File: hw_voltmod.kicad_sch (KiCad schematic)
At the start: 10 parts, among them J101 Conn_01x09_Pin, U104 L78L33_SO8

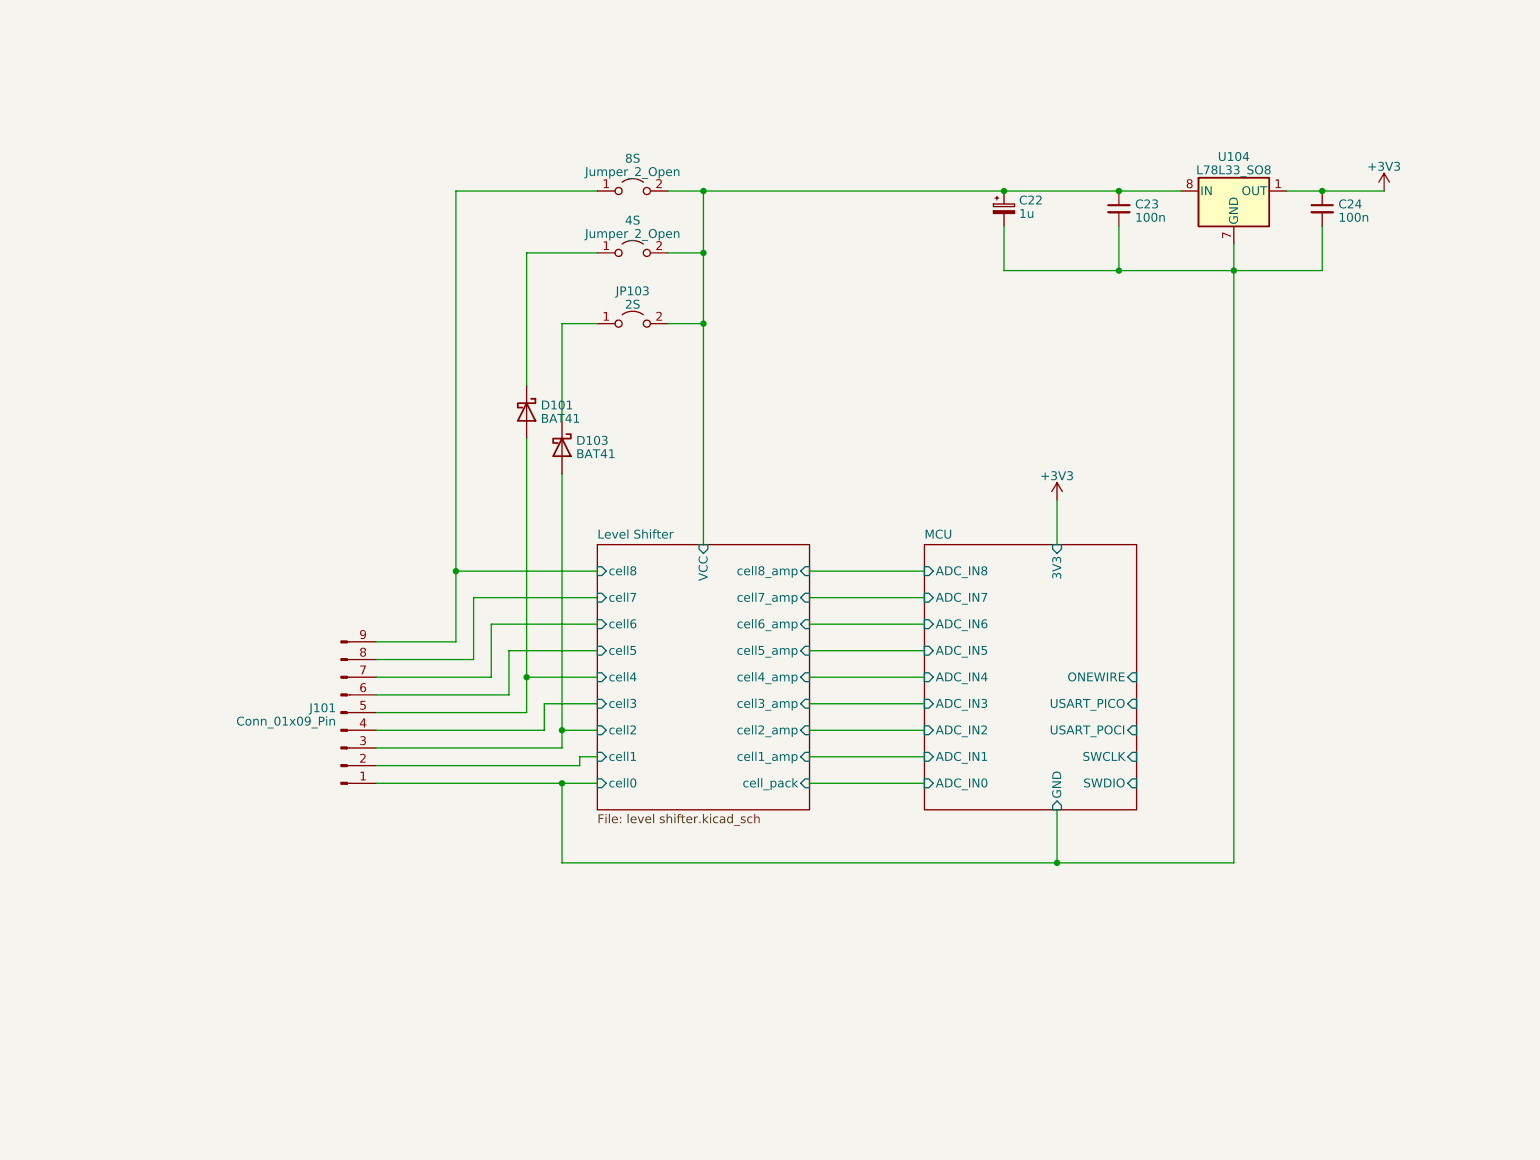
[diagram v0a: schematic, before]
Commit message: asdf
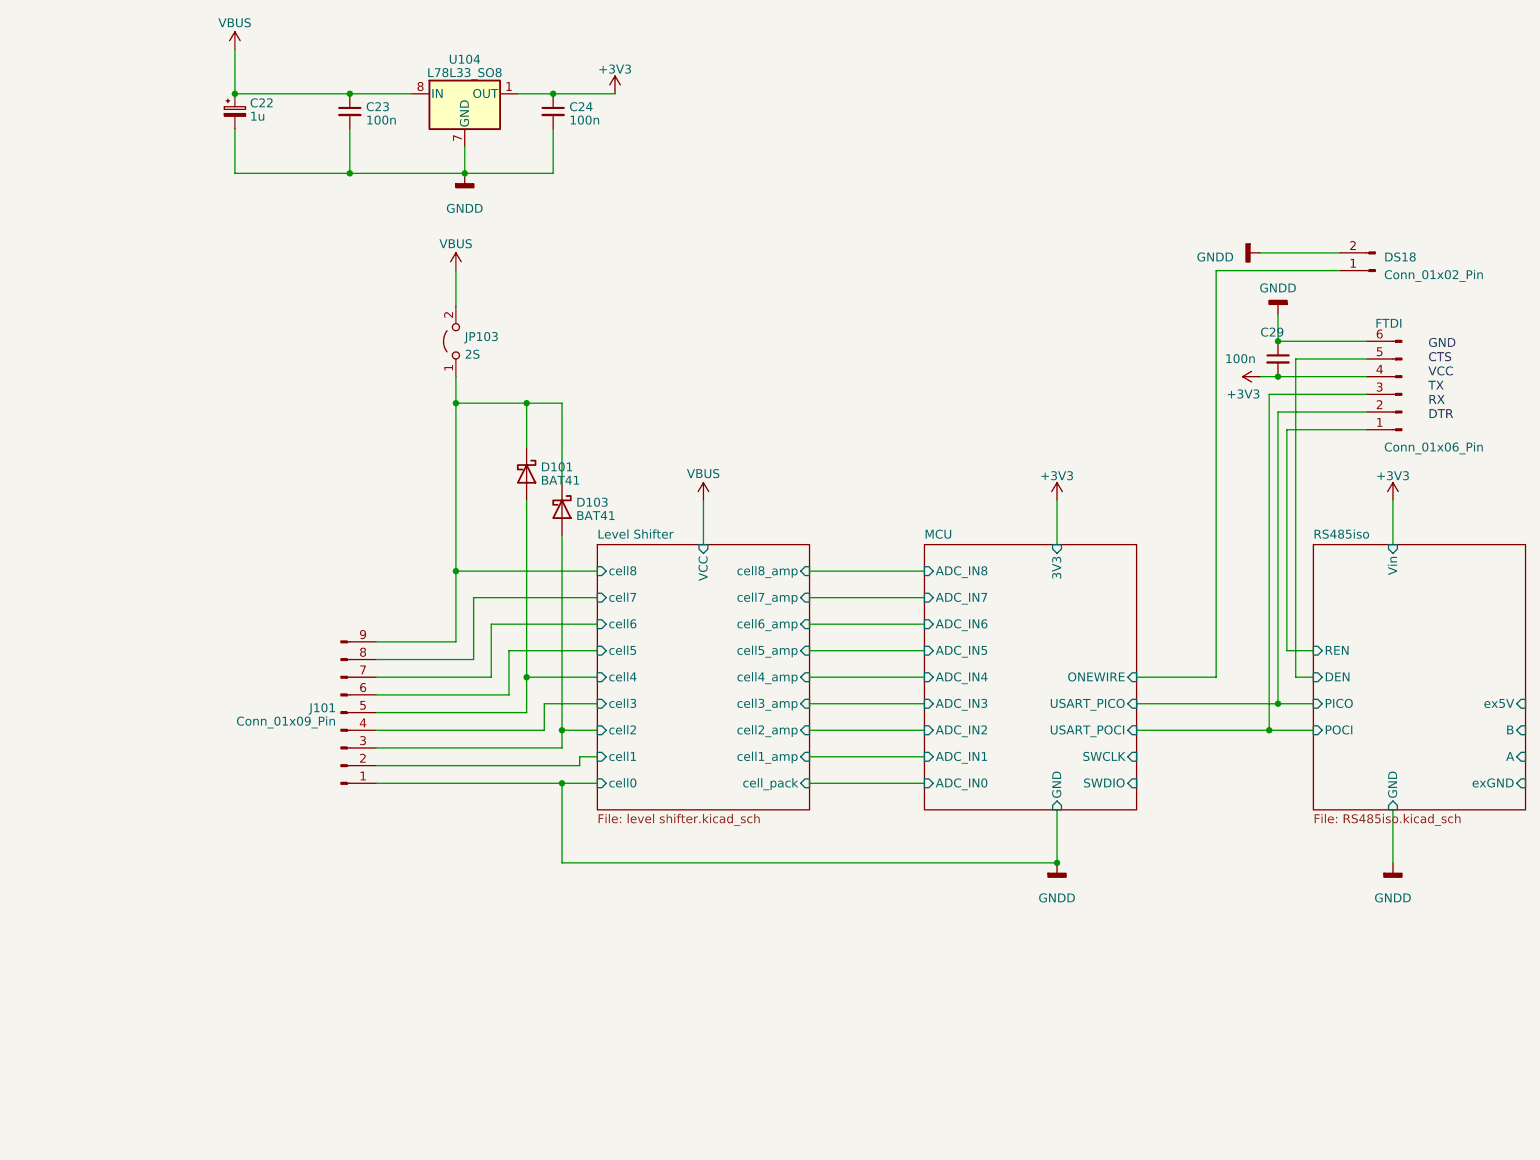
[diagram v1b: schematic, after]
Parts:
- removed 4S, 8S: Jumper_2_Open, symbol Jumper:Jumper_2_Open
- added C29: 100n, Capacitor_SMD:C_0603_1608Metric_Pad1.08x0.95mm_HandSolder, symbol Device:C_Small
- added DS18: Conn_01x02_Pin, symbol Connector:Conn_01x02_Pin
- added FTDI: Conn_01x06_Pin, symbol Connector:Conn_01x06_Pin
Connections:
- net +3V3: now also C29.2, FTDI.4 (Pin_4)
- net Level Shifter/cell8: now also D101.1 (K), D103.1 (K), JP103.1 (A)
- net MCU/ONEWIRE: now also DS18.1 (Pin_1)
- net MCU/USART_PICO: now also FTDI.2 (Pin_2)
- net MCU/USART_POCI: now also FTDI.3 (Pin_3)
- net Level Shifter/VCC renamed VBUS
- net Level Shifter/cell0 renamed GNDD
- net GNDD: now also C29.1, DS18.2 (Pin_2), FTDI.6 (Pin_6)
- new net RS485iso/DEN: FTDI.5 (Pin_5)
- new net RS485iso/REN: FTDI.1 (Pin_1)
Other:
- added sheet RS485iso (RS485iso.kicad_sch)
- note added: "GND CTS VCC TX RX DTR"
- moved on the sheet: C22, C23, C24, D101, D103, U104

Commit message: asdf
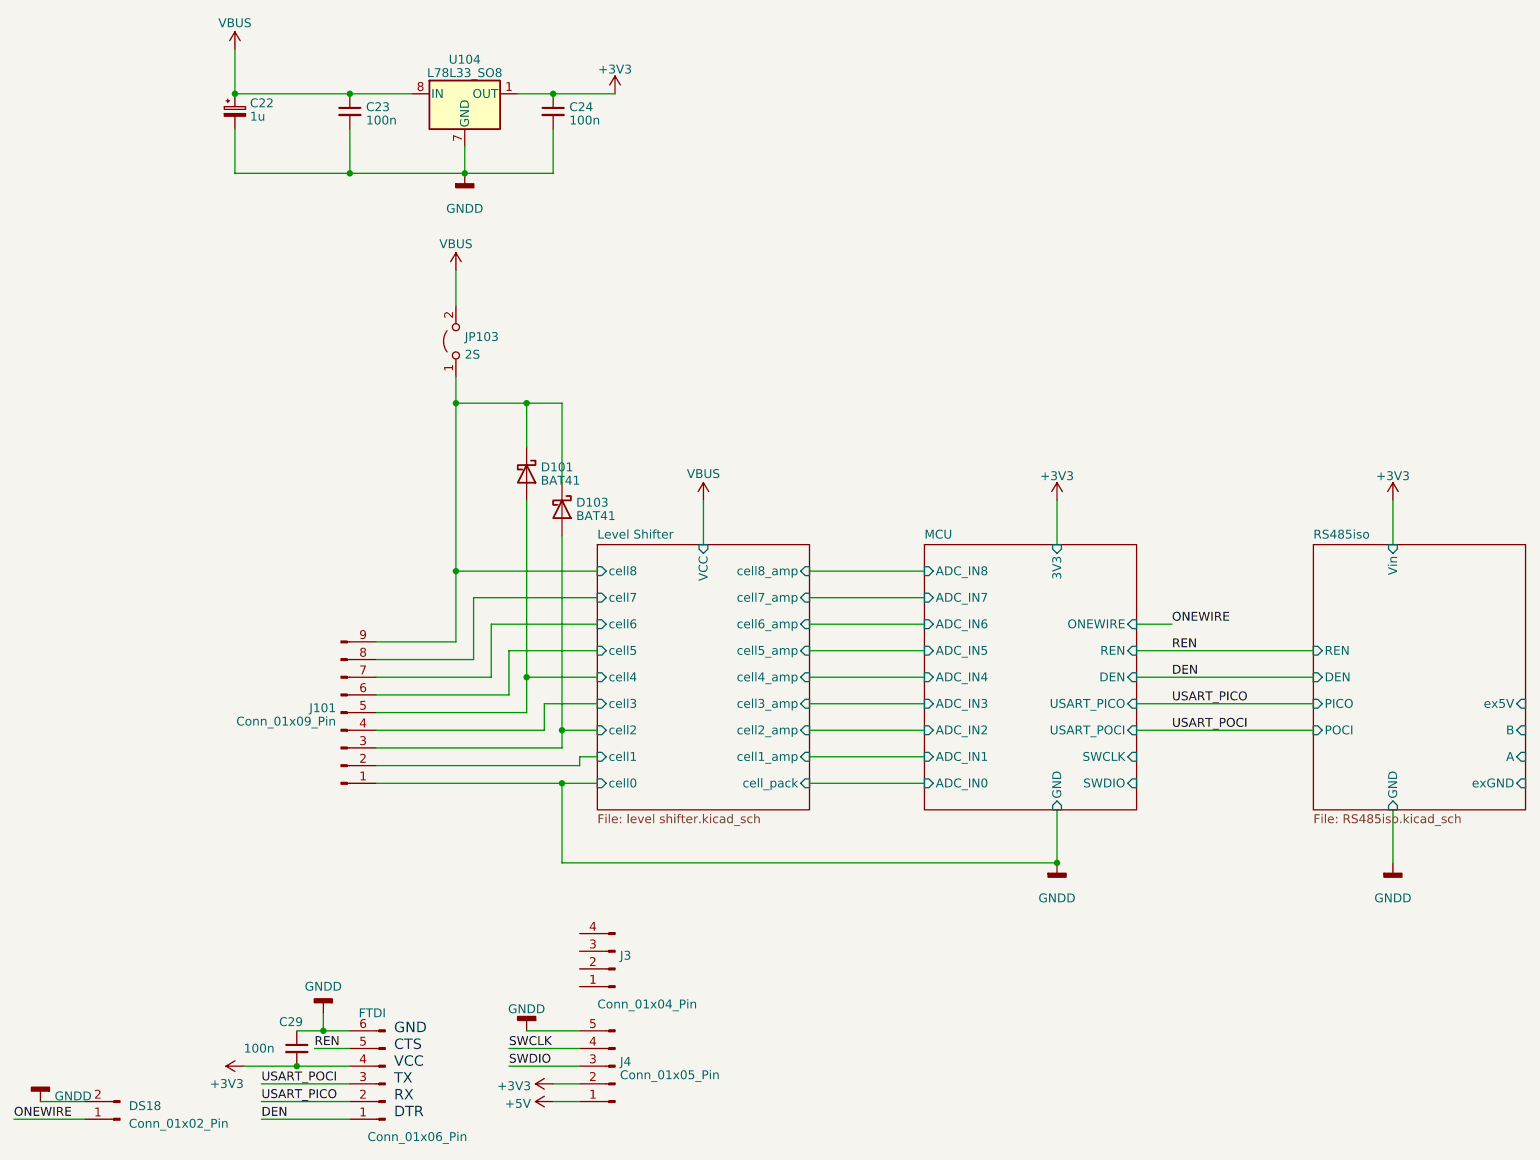
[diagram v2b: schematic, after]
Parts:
- added J3: Conn_01x04_Pin, symbol Connector:Conn_01x04_Pin
- added J4: Conn_01x05_Pin, symbol Connector:Conn_01x05_Pin
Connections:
- net +3V3: now also J4.2 (Pin_2)
- net GNDD: now also J4.5 (Pin_5)
- net MCU/ONEWIRE renamed ONEWIRE
- net MCU/USART_PICO renamed USART_PICO
- net MCU/USART_POCI renamed USART_POCI
- net RS485iso/DEN renamed REN
- net RS485iso/REN renamed DEN
- new net +5V: J4.1 (Pin_1)
- new net SWCLK: J4.4 (Pin_4)
- new net SWDIO: J4.3 (Pin_3)
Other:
- sheet MCU ports: added DEN, REN; removed none
- moved on the sheet: C29, DS18, FTDI
